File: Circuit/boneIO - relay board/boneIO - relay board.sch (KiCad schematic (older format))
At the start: 70 parts, among them J1 Screw_Terminal_01x04, J10 Screw_Terminal_01x04, J11 Screw_Terminal_01x04, J2 Screw_Terminal_01x04, J3 Conn_02x13_Odd_Even, J4 Screw_Terminal_01x04, J5 Screw_Terminal_01x04, J6 Screw_Terminal_01x04, J7 Screw_Terminal_01x04, J8 Screw_Terminal_01x04, J9 Screw_Terminal_01x04, K1 RM85-2011-35-1005, K10 RM85-2011-35-1005, K11 RM85-2011-35-1005, K12 RM85-2011-35-1005, K13 RM85-2011-35-1005, K14 RM85-2011-35-1005, K15 RM85-2011-35-1005, K16 RM85-2011-35-1005, K17 RM85-2011-35-1005, K18 RM85-2011-35-1005, K19 RM85-2011-35-1005, K2 RM85-2011-35-1005, K20 RM85-2011-35-1005, K3 RM85-2011-35-1005, K4 RM85-2011-35-1005, K5 RM85-2011-35-1005, K6 RM85-2011-35-1005, K7 RM85-2011-35-1005, K8 RM85-2011-35-1005, K9 RM85-2011-35-1005, U1 MCP9808_MSOP, U2 ULN2803A, U3 ULN2803A, U4 ULN2803A

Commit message: Repo Sync for new people
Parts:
- removed C1: 100n, Capacitor_SMD:C_0603_1608Metric, symbol Device:C
- removed C2, C3, C4: 4.7uF/50V, Capacitor_SMD:C_1206_3216Metric, symbol Device:C
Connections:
- wire segments 401 -> 393
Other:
- note removed: "OPTIONAL"
- moved on the sheet: R1, R2, R3, R4, R5, R6, R7, R8, R9

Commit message: Wykonana PCB RELAY RM85_v0.2
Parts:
- removed H1, H2: MountingHole, MountingHole:MountingHole_4.3mm_M4, symbol Mechanical:MountingHole
- removed J3: Conn_02x13_Odd_Even, Connector_PinHeader_2.54mm:PinHeader_2x13_P2.54mm_Vertical, symbol Connector_Generic:Conn_02x13_Odd_Even
- removed R1, R3, R5: 0k, Resistor_SMD:R_0603_1608Metric, symbol Device:R
- removed R14, R15, R16, R17, R18, R19, R20, R21, R22, R23, R24, R25, R26, R27, R28, R29: 10k, Resistor_SMD:R_0603_1608Metric, symbol Device:R
- added C1, C2, C3, C4, C5, C6: 100n, Capacitor_SMD:C_0603_1608Metric, symbol Device:C
- added J12, J13: Screw_Terminal_01x04, Connector_Phoenix_GMSTB:PhoenixContact_GMSTBA_2,5_4-G_1x04_P7.50mm_Horizontal, symbol Connector:Screw_Terminal_01x04
- added J3: Conn_02x04_Odd_Even, Connector_PinSocket_2.54mm:PinSocket_2x04_P2.54mm_Vertical, symbol Connector_Generic:Conn_02x04_Odd_Even
- added K21, K22, K23, K24: RM85-2011-35-1005, boneIO - RM85:RM852011351005_1, symbol boneIO---relay-board-rescue:RM85-2011-35-1005-MK-boneIO---relay-board-rescue
- added R7: 4.7k, Resistor_SMD:R_0603_1608Metric, symbol Device:R
- added R8, R9: 0k, Resistor_SMD:R_0603_1608Metric, symbol Device:R
- added SW1, SW2, SW3: SW_DIP_x03, Button_Switch_SMD:SW_DIP_SPSTx03_Slide_KingTek_DSHP03TJ_W5.25mm_P1.27mm_JPin, symbol Switch:SW_DIP_x03
- added U2, U3: MCP23017_SS, Package_SO:SSOP-28_5.3x10.2mm_P0.65mm, symbol Interface_Expansion:MCP23017_SS
- K1, K10, K11, K12, K13, K14, K15, K16, K17, K18, K19, K2, K20, K3, K4, K5, K6, K7, K8, K9: footprint RM85-2011-35-1005:RM852011351005 -> boneIO - RM85:RM852011351005_1; symbol boneIO---relay-board-rescue:RM85-2011-35-1005-MK -> boneIO---relay-board-rescue:RM85-2011-35-1005-MK-boneIO---relay-board-rescue
- R10, R11, R12, R13: value 10k -> 0k
- U1: symbol Sensor_Temperature:MCP9808_MSOP -> boneIO---relay-board-rescue:MCP9808_MSOP-Sensor_Temperature-boneIO---relay-board-rescue
- renumbered R2 to R1, R7 to R2, R4 to R3, R6 to R4, R8 to R5, R9 to R6, U2 to U4, U3 to U5, U4 to U6
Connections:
- net labels added: +3.3V, +5V, K21, K22, K23, K24, RELAY21, RELAY22, RELAY23, RELAY24, RESET_MCP
- wire segments 393 -> 477
- no-connect marks 80 -> 52
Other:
- moved on the sheet: J1, J10, J11, J2, J4, J5, J6, J7, J8, J9, R1, R2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

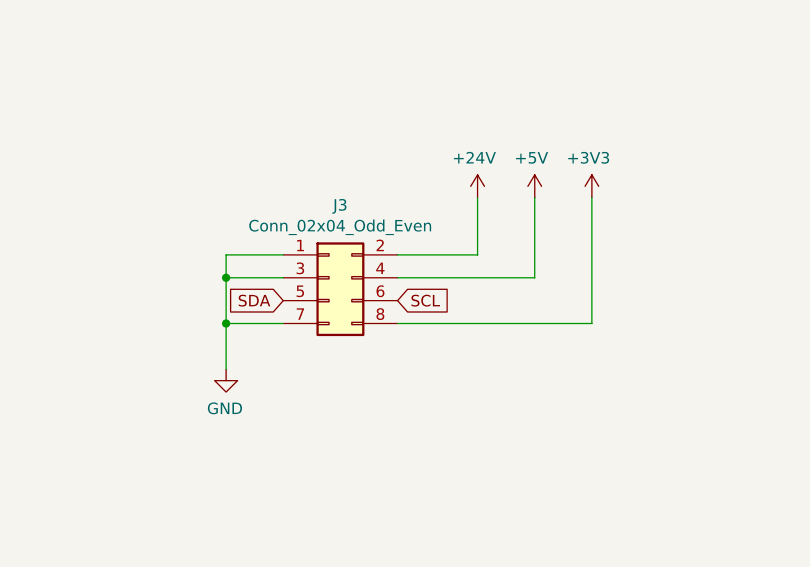
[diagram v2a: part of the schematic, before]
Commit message: 01.11.2021
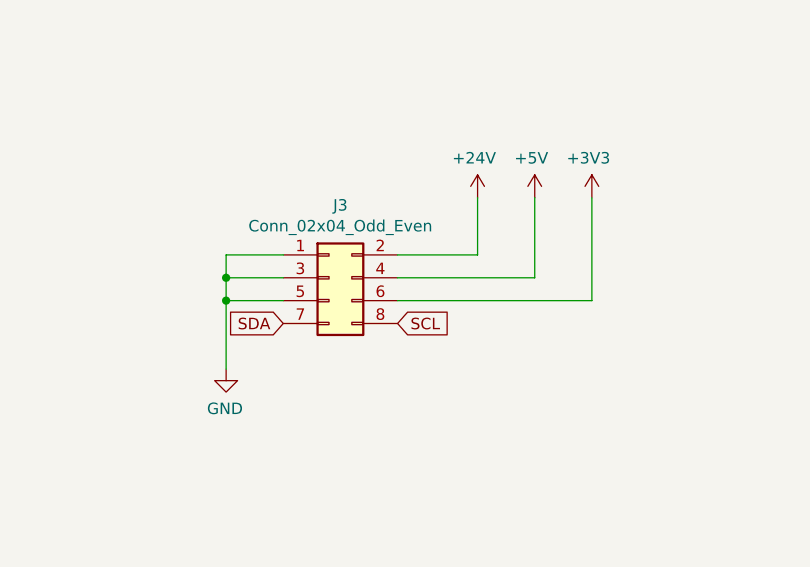
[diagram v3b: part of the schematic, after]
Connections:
- net +3V3: now also J3.6 (Pin_6); no longer J3.8 (Pin_8)
- net GND: now also J3.5 (Pin_5); no longer J3.7 (Pin_7)
- net SCL: now also J3.8 (Pin_8); no longer J3.6 (Pin_6)
- net SDA: now also J3.7 (Pin_7); no longer J3.5 (Pin_5)
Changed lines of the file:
@@
 	8900 3950 8300 3950
 Wire Wire Line
-	9150 3600 9150 4150
-Wire Wire Line
-	9150 4150 8300 4150
-Wire Wire Line
-	7550 4350 7550 4150
+	9150 3600 9150 4050
+Wire Wire Line
+	9150 4050 8300 4050
 Wire Wire Line
 	7550 3850 7800 3850
@@
 	7550 3950 7550 3850
 Wire Wire Line
-	7800 4150 7550 4150
-Connection ~ 7550 4150
-Wire Wire Line
-	7550 4150 7550 3950
-Text GLabel 8300 4050 2    50   Input ~ 0
+	7800 4050 7550 4050
+Text GLabel 8300 4150 2    50   Input ~ 0
 SCL
-Text GLabel 7800 4050 0    50   Input ~ 0
+Text GLabel 7800 4150 0    50   Input ~ 0
 SDA
 $Comp
@@
 Text GLabel 10500 -1850 0    50   Input ~ 0
 RESET_MCP
+Wire Wire Line
+	7550 3950 7550 4050
+Connection ~ 7550 4050
+Wire Wire Line
+	7550 4050 7550 4350
 $EndSCHEMATC
